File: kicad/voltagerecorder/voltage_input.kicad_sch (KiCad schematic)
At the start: 11 parts

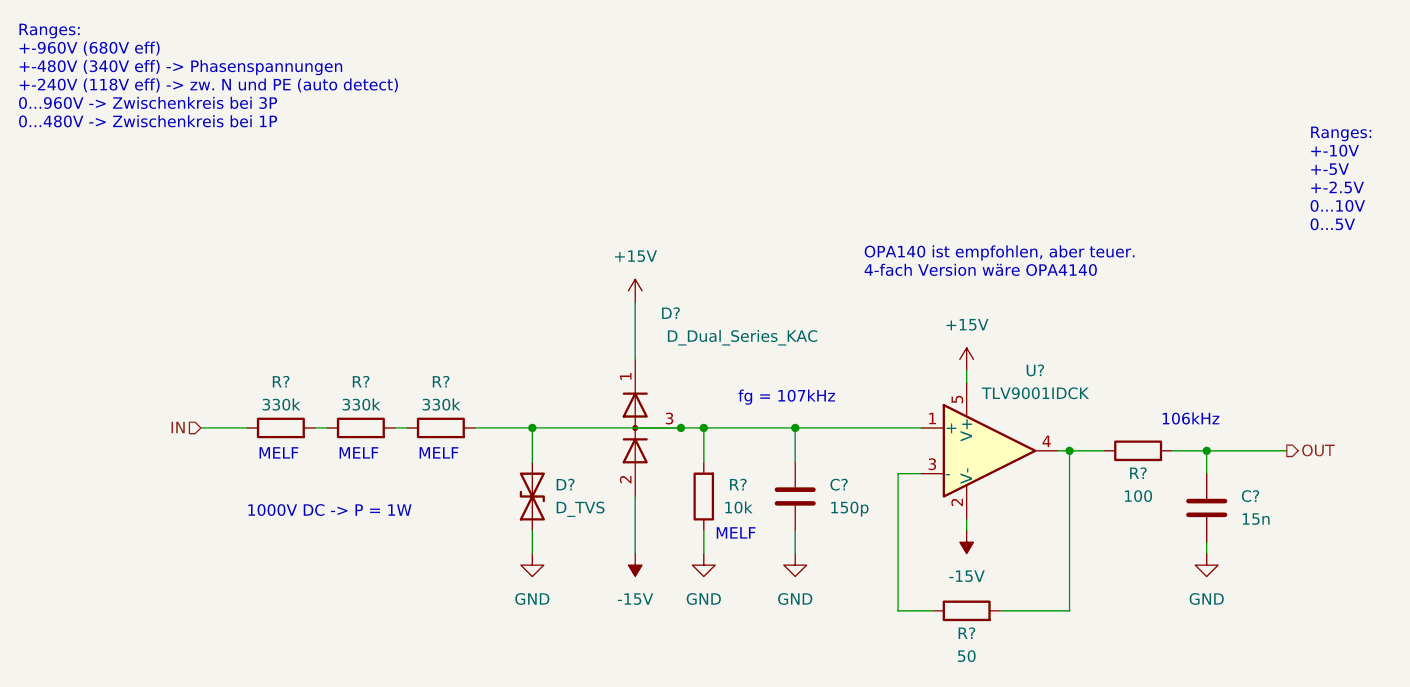
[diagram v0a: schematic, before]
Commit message: a
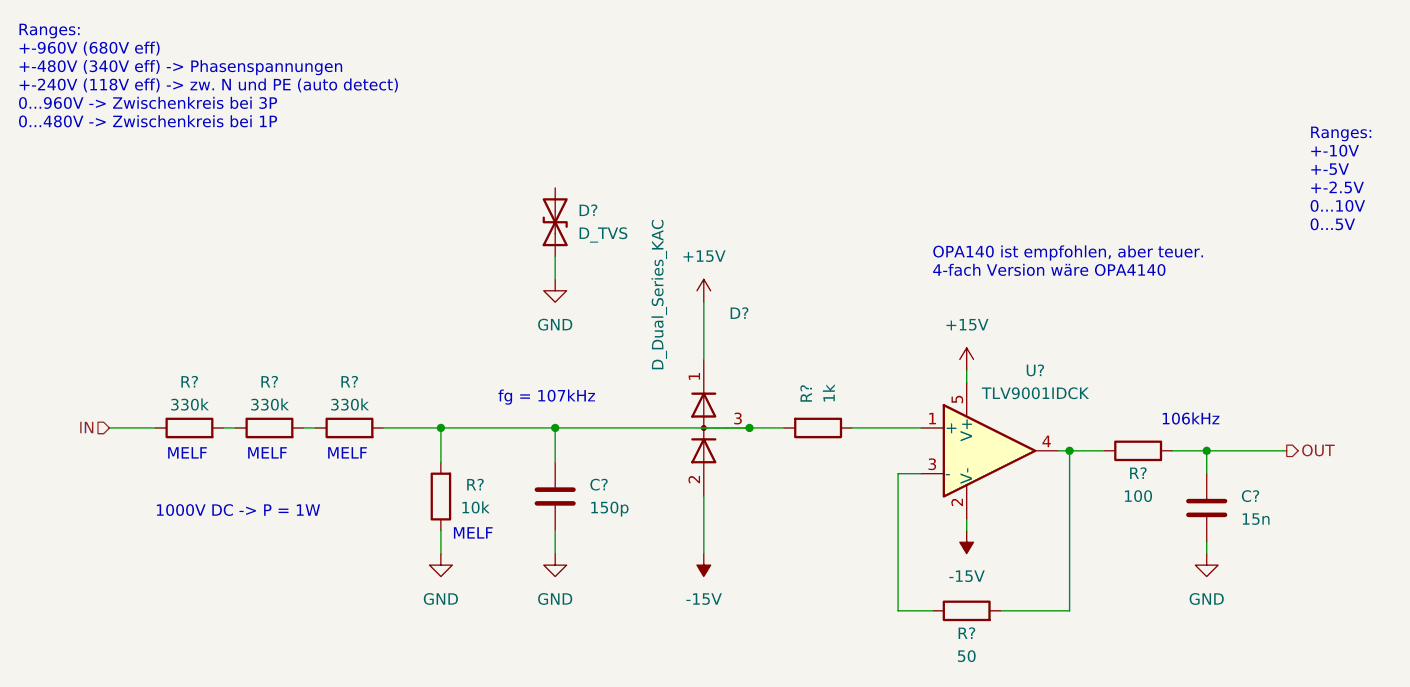
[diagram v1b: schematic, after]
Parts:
- added R?: 1k, symbol Device:R
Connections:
- net at C?.1, D?.3 (common), R?.2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: now also R?.2; no longer D?.2 (A2), U?.1 (+)
- new net: R?.1, U?.1 (+)
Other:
- moved on the sheet: C?, D?, R?
